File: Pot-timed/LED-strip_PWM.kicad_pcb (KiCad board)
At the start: 2 copper layers, 29.7 x 10 mm, 16 parts, among them IC1 MADW__ATTINY13-MM, P1 CONN_2, P2 CONN_2, T1 AO3400, U1 MCP1804-SOT23-5

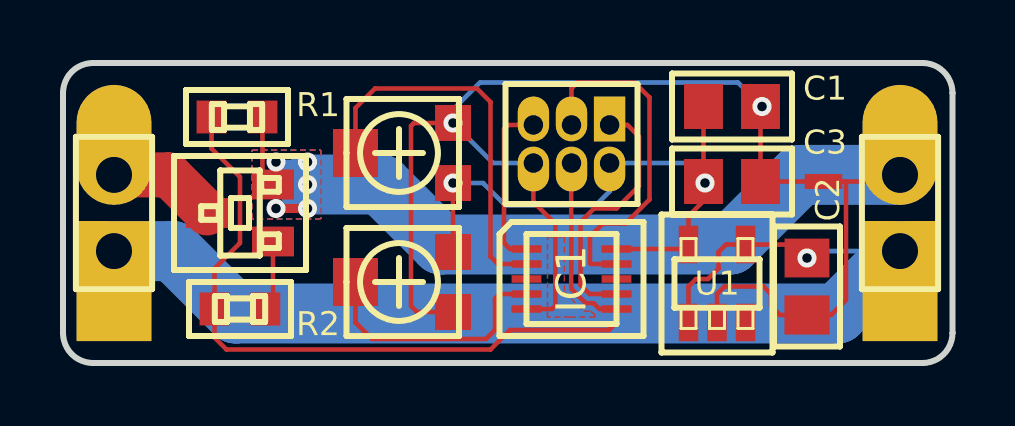
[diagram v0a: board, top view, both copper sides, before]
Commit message: Pot-timed (single board): switched to ATtiny10 SOT23-6.
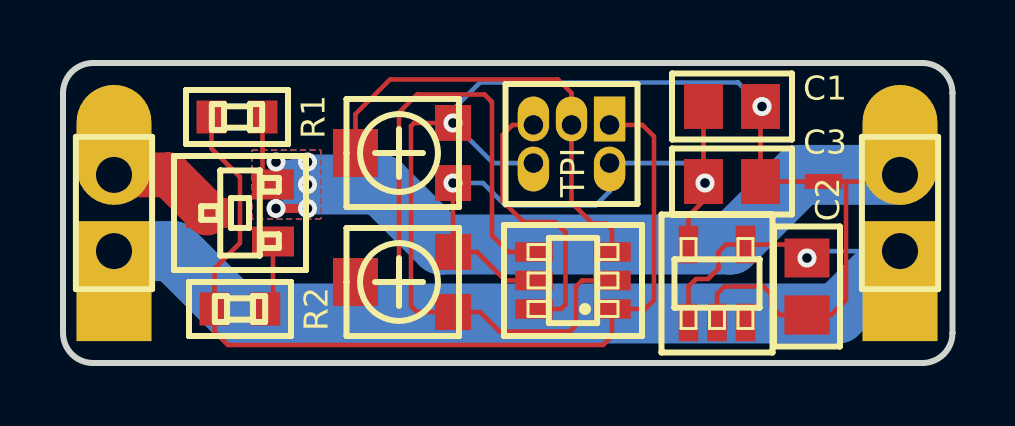
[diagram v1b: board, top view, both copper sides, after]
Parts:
- IC1: value MADW__ATTINY13-MM -> ATTINY10-TS; footprint MADW__MLF10 -> MADW__SOT23-6
- JP1: value ISP -> TPI
- moved IC1 0.07 mm to (93.0, 55.2), turned to 90 degrees
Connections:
- IC1 pad 1: /RESET -> /GATE
- IC1 pad 2: /POT1 -> GND
- IC1 pad 3: N-000005 -> /POT1
- IC1 pad 5: GND -> VCC
- IC1 pad 6: /MOSI -> /RESET
- JP1 pad 1: /MISO -> /GATE
- JP1 pad 3: /SCK -> /POT1
- R1 pad 2: /MOSI -> /GATE
- R2 pad 1: /MOSI -> /GATE
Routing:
- net /GATE: track 0.00 -> 31.7 mm
- net /MOSI: track 29.2 -> 0.00 mm
- net /SCK: track 11.8 -> 0.00 mm
- net /MISO: track 8.66 -> 0.00 mm
- net /POT2: track 8.51 -> 16.5 mm
- net /RESET: track 5.67 -> 9.42 mm
- net /POT1: track 12.9 -> 15.3 mm
- net GND: track 34.1 -> 35.1 mm
- net VCC: track 20.0 -> 20.6 mm
- removed copper zone on F.Cu, net GND
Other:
- board text added: "V0.13 POT PWM controller"
- board text removed: "V0.12 POT PWM controller"

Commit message: Revert "Pot-timed (single board): switched to ATtiny10 SOT23-6."
This reverts commit c61ef78eb5273ce0300997b1b0118eed30148325.

C + ATtiny10 not supported by avr-gcc
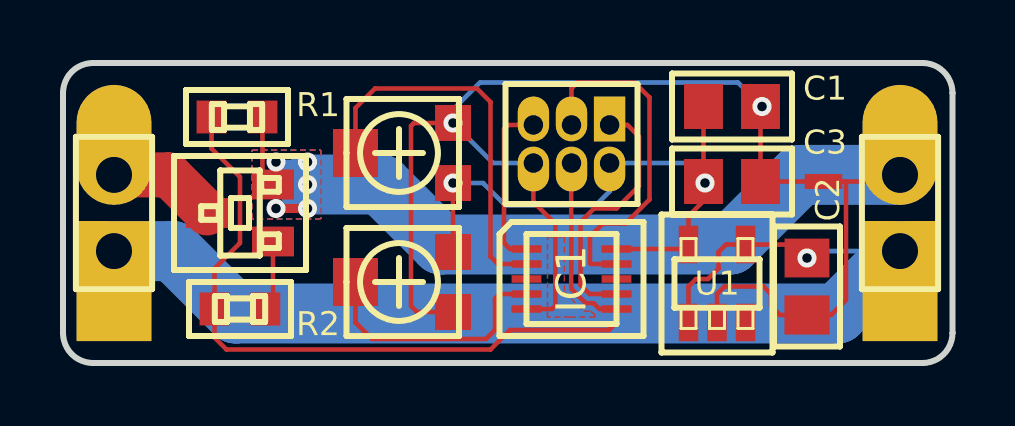
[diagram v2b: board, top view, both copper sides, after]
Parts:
- IC1: value ATTINY10-TS -> MADW__ATTINY13-MM; footprint MADW__SOT23-6 -> MADW__MLF10
- JP1: value TPI -> ISP
- moved IC1 0.07 mm to (93.0, 55.2), turned to 0 degrees
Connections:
- IC1 pad 1: /GATE -> /RESET
- IC1 pad 2: GND -> /POT1
- IC1 pad 3: /POT1 -> N-000005
- IC1 pad 5: VCC -> GND
- IC1 pad 6: /RESET -> /MOSI
- JP1 pad 1: /GATE -> /MISO
- JP1 pad 3: /POT1 -> /SCK
- R1 pad 2: /GATE -> /MOSI
- R2 pad 1: /GATE -> /MOSI
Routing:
- net /GATE: track 31.7 -> 0.00 mm
- net /MOSI: track 0.00 -> 29.2 mm
- net /SCK: track 0.00 -> 11.8 mm
- net /MISO: track 0.00 -> 8.66 mm
- net /POT2: track 16.5 -> 8.51 mm
- net /RESET: track 9.42 -> 5.67 mm
- net /POT1: track 15.3 -> 12.9 mm
- net GND: track 35.1 -> 34.1 mm
- net VCC: track 20.6 -> 20.0 mm
- added copper zone on F.Cu, net GND
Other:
- board text added: "V0.12 POT PWM controller"
- board text removed: "V0.13 POT PWM controller"
